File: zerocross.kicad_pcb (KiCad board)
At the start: 2 copper layers, 31 x 21 mm, 16 parts, among them J1 OUTPUT, J2 INPUT, Q1 BC847, Q2 BC847, U1 PC817

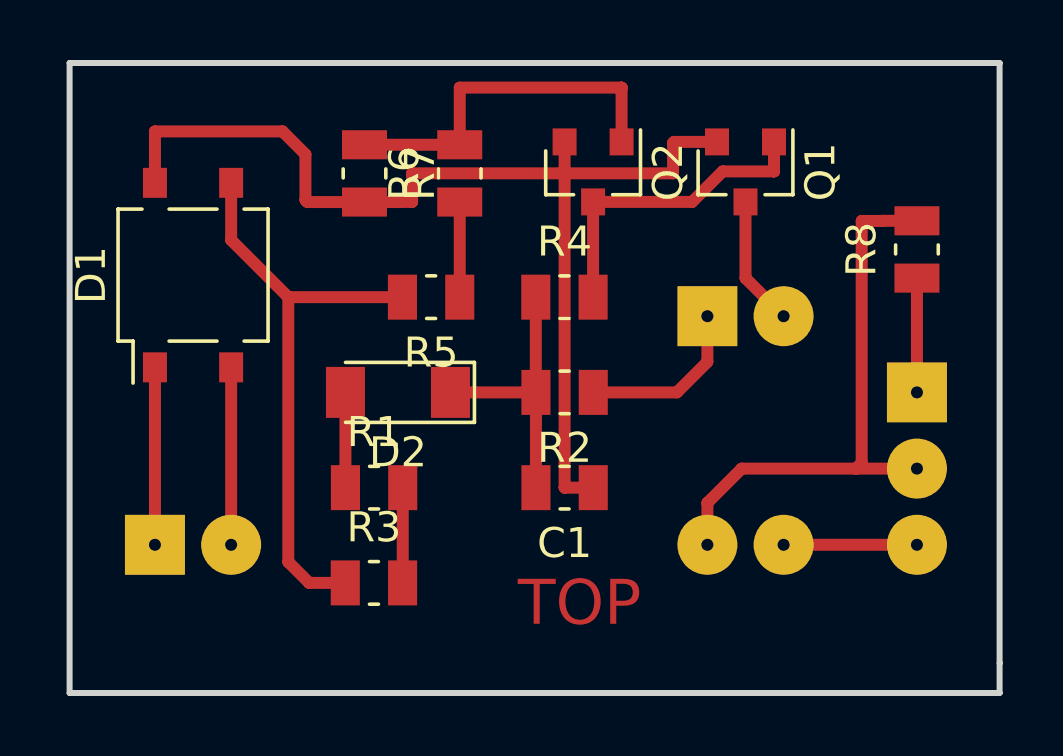
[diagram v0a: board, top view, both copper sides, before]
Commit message: Solder
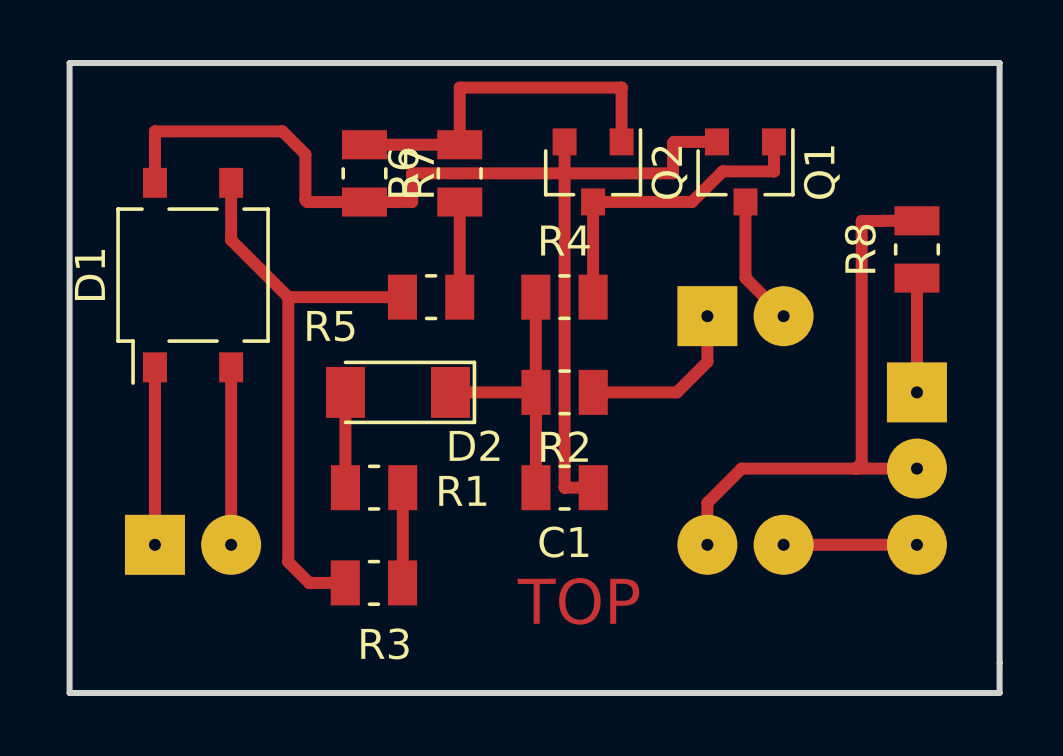
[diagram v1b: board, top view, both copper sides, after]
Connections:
- net Net-(D1-Pad3) renamed /+
